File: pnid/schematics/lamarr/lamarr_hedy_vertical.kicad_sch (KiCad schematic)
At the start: 103 parts, among them U1 Rocket_Big

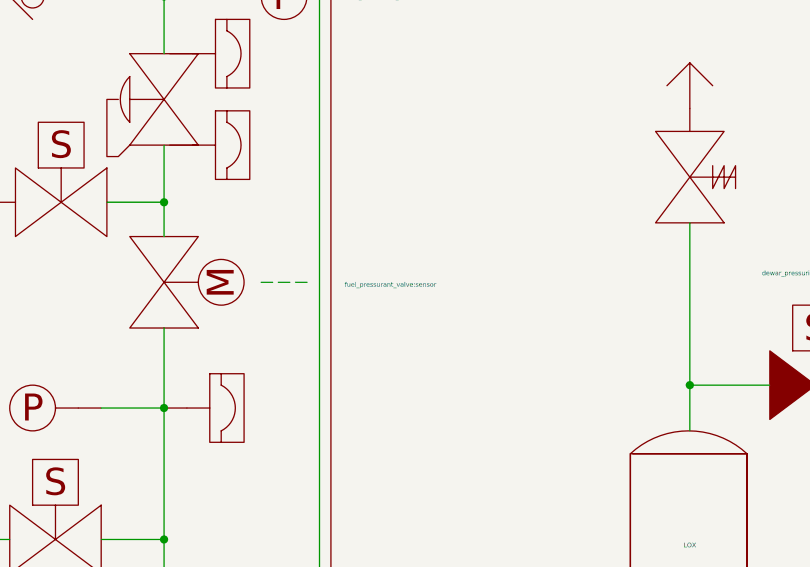
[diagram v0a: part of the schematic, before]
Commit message: label position again
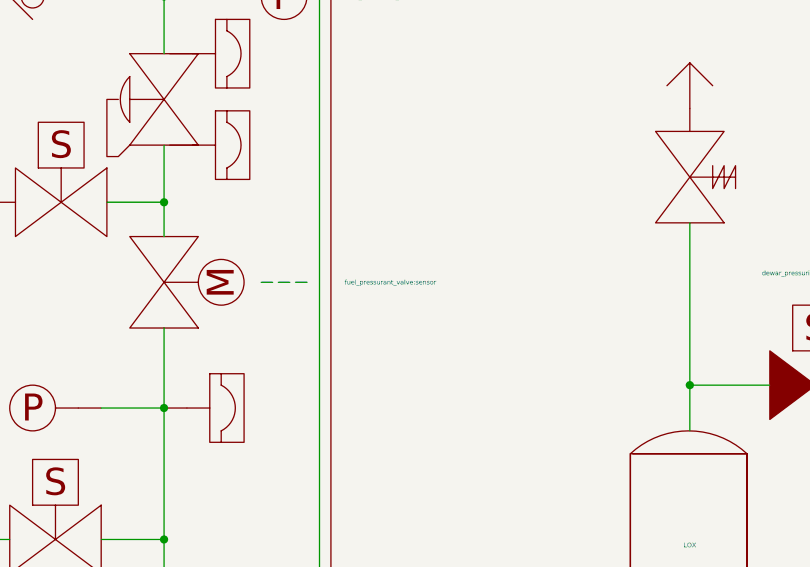
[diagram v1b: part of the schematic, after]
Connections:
- net at engine.~ (C): now also venturi1.~
- net at ox_venturi.~: now also ox_main_valve.~, ox_venturi_pressure.~; no longer engine.~ (C)
- net at venturi1.~: now also fuel_main_valve.~, fuel_venturi_pressure.~; no longer engine.~ (C)
- net at dewar_needle_valve?.~: now also C2.~, C3.~, press_in.~; no longer C1.~
- new net: engine.~ (C), ox_venturi.~
- new net: OX.~, ox_main_valve.~, ox_quick_connect.~
- new net: DewarOverPressureValve?.~, LOX.~, dewar_pressurize_solenoid.~
- new net: C1.~, dewar_needle_valve?.~
- new net: ox_pressurant_valve.~, ox_pressurant_vent_valve.~, pressurantPressureRegulator2.~
- new net: FUEL.~, fuel_main_valve.~, ox_quick_connect1.~
- new net: fuel_pressurant_valve.~, fuel_pressurant_vent_valve.~, pressurantPressureRegulator1.~
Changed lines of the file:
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@@
 		)
 		(property "Value" "fuel_pressurant_valve:sensor"
-			(at 87.376 71.374 90)
+			(at 87.376 71.12 90)
 			(effects
 				(font
